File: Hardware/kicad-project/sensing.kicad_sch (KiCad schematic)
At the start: 34 parts, among them U1 LM358P, U2 LEM-CAS-6NP, U3 LM358P, U4 LM358P

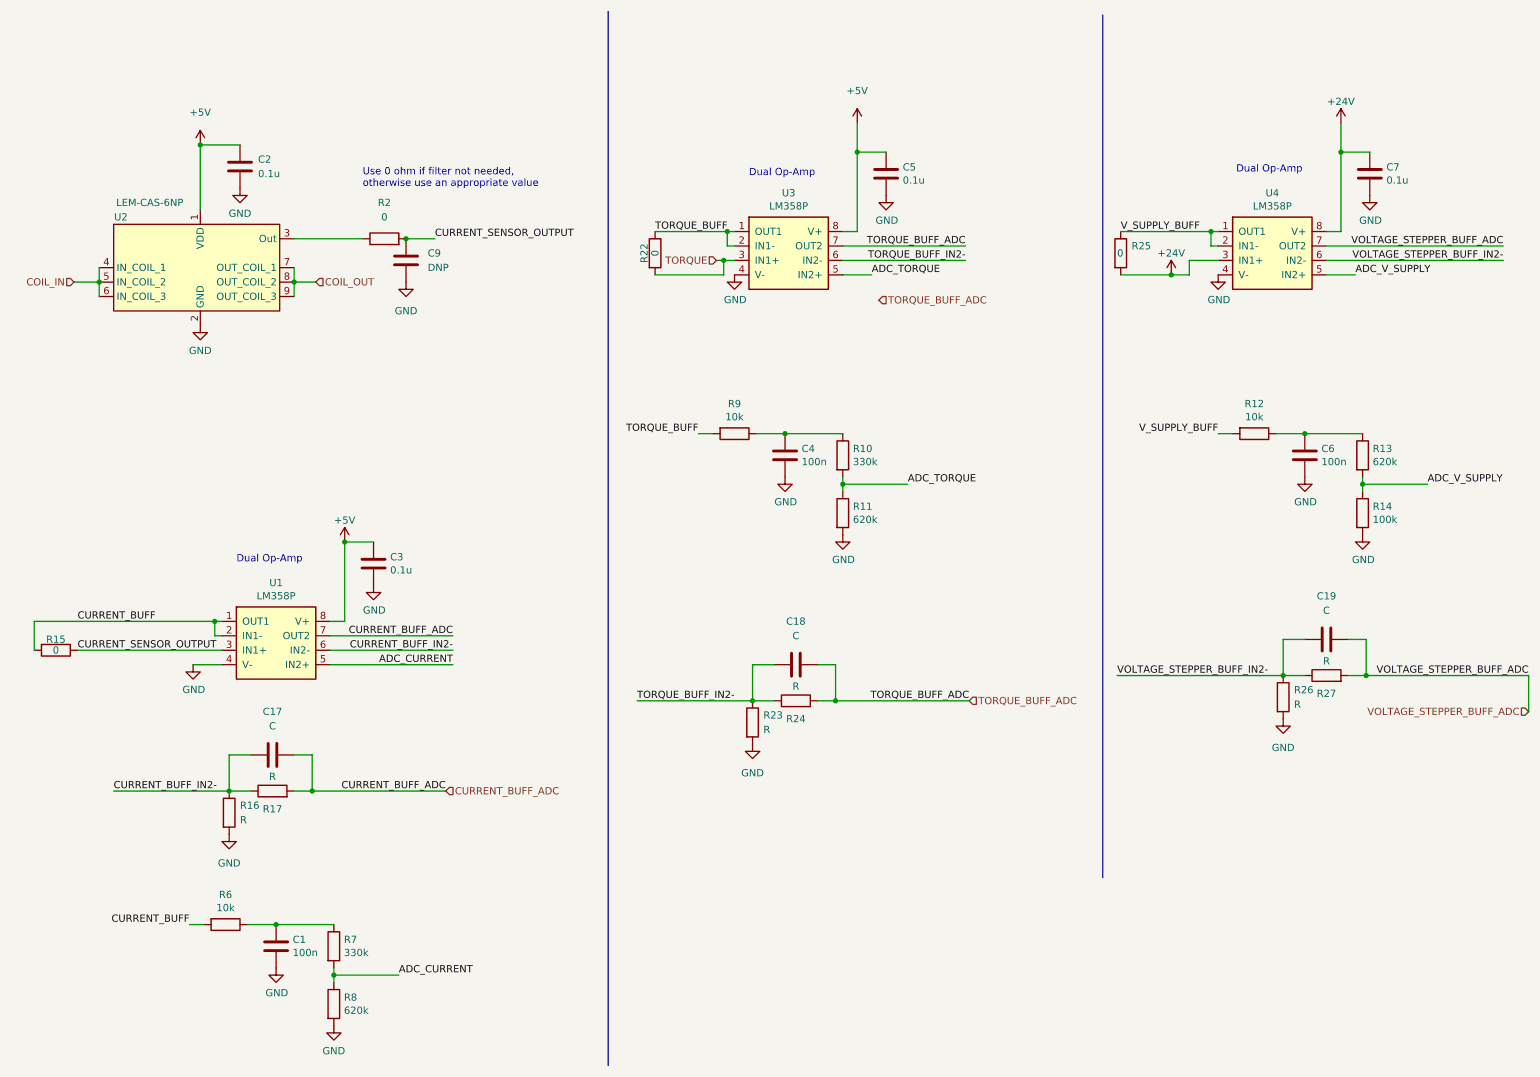
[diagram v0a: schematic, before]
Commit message: hw: final pdf schematic upload
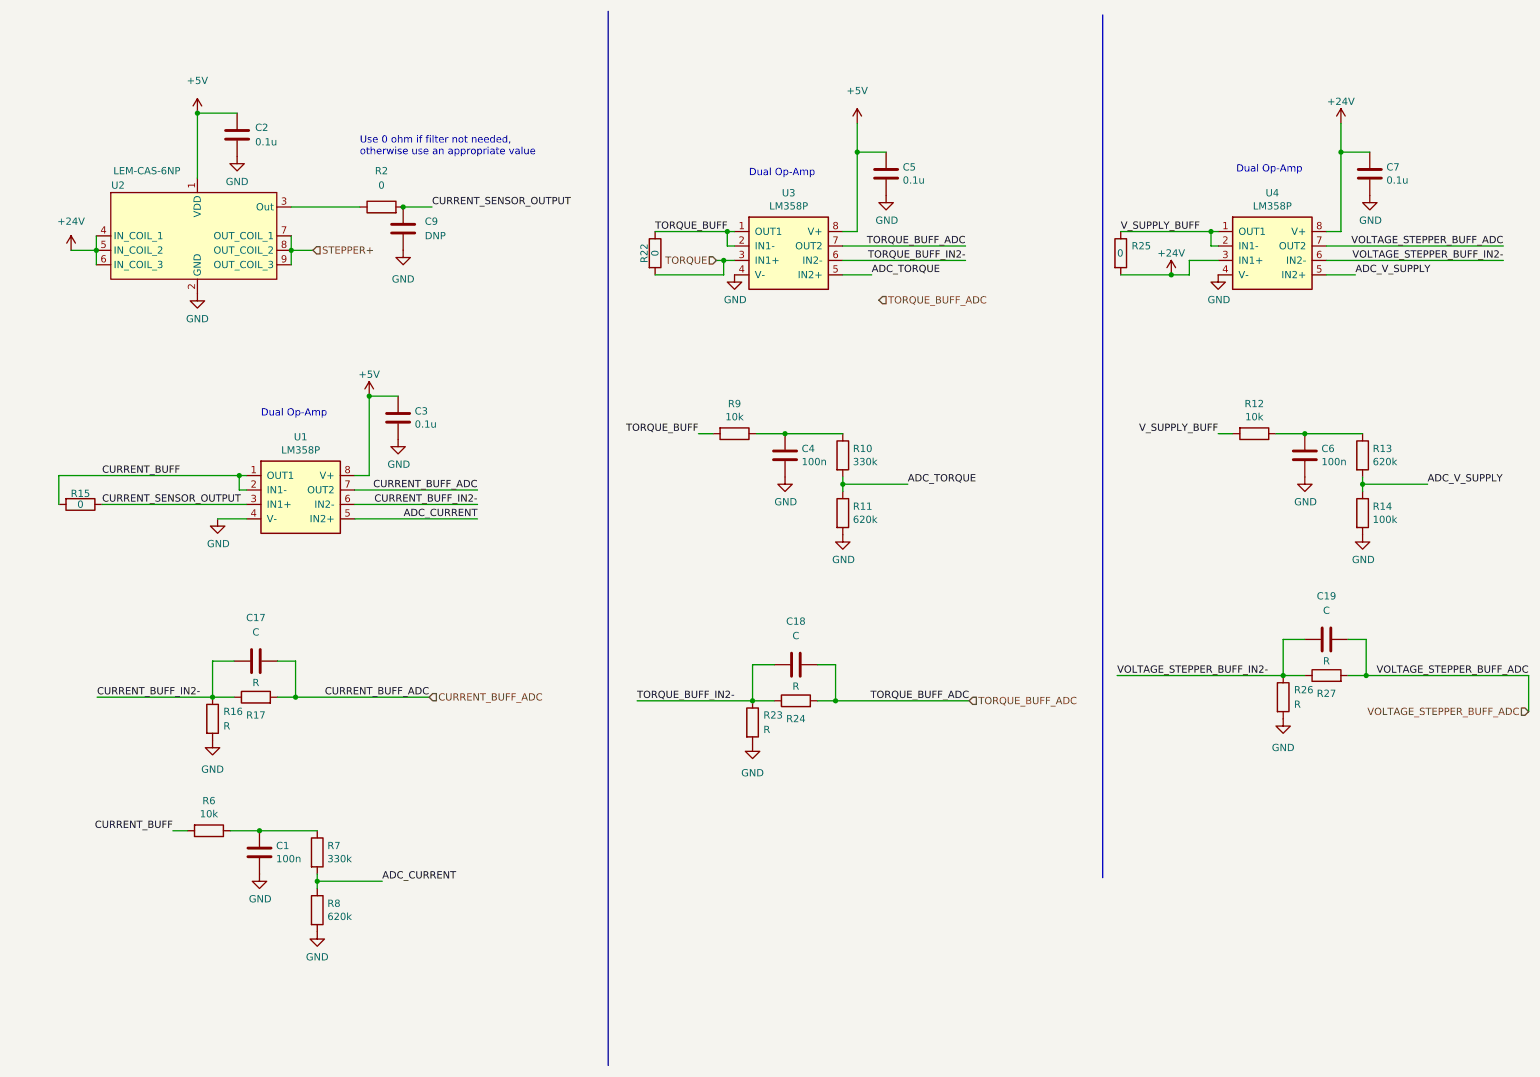
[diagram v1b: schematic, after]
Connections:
- net COIL_IN is gone; now on net +24V: U2.4 (IN_COIL_1), U2.5 (IN_COIL_2), U2.6 (IN_COIL_3)
- net COIL_OUT renamed STEPPER+
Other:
- moved on the sheet: C1, C17, C2, C3, C9, R15, R16, R17, R2, R6, R7, R8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
